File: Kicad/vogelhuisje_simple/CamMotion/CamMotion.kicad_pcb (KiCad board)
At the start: 2 copper layers, 91.4 x 137.2 mm, 20 parts, among them J6 Conn_01x21_Female, P2 GenericBoostConverter, P3 TP4056breakout, P4 TP4056breakout, Q1 Q_PMOS_GSD, U3 ESP32-LilyGo-T_PCIE, U4 PMS5003, U5 SD-card-reader, U6 BME280Breakout, U7 BME280Breakout

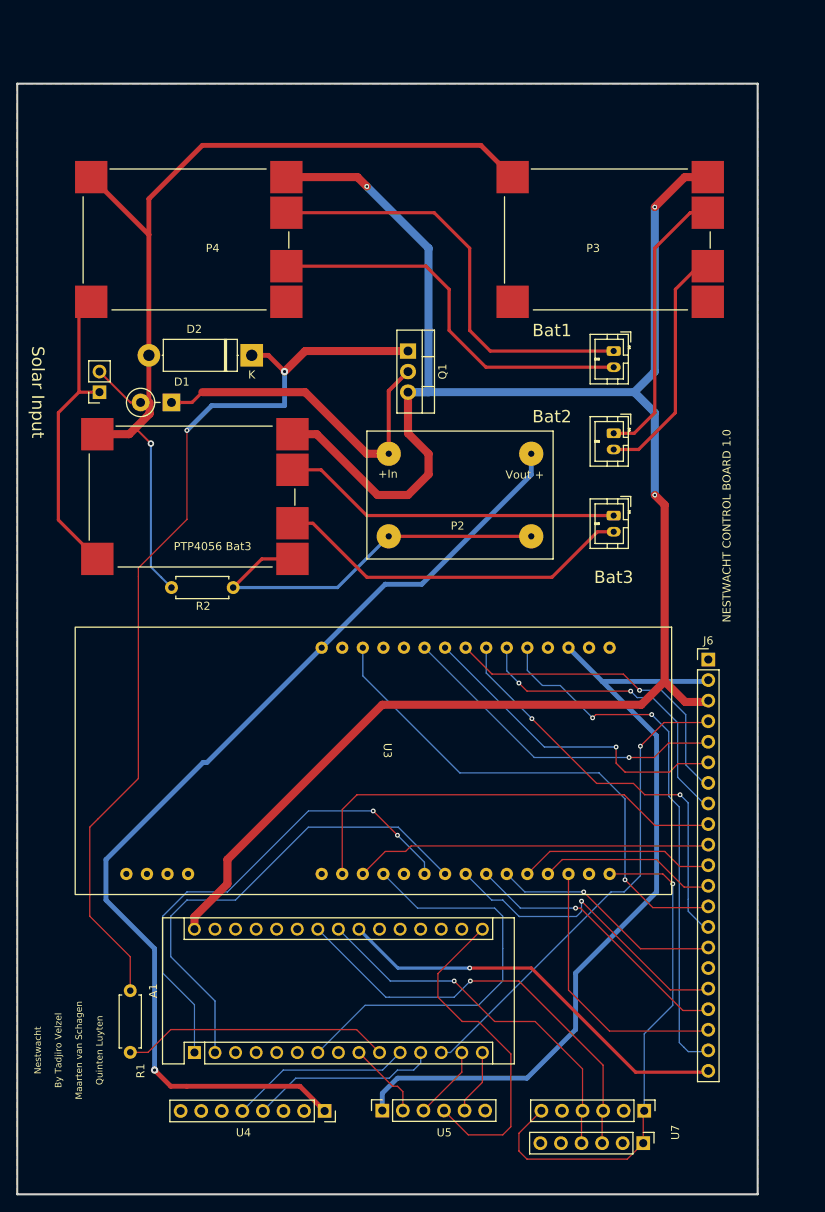
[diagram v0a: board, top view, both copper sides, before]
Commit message: Finish pcb simplified
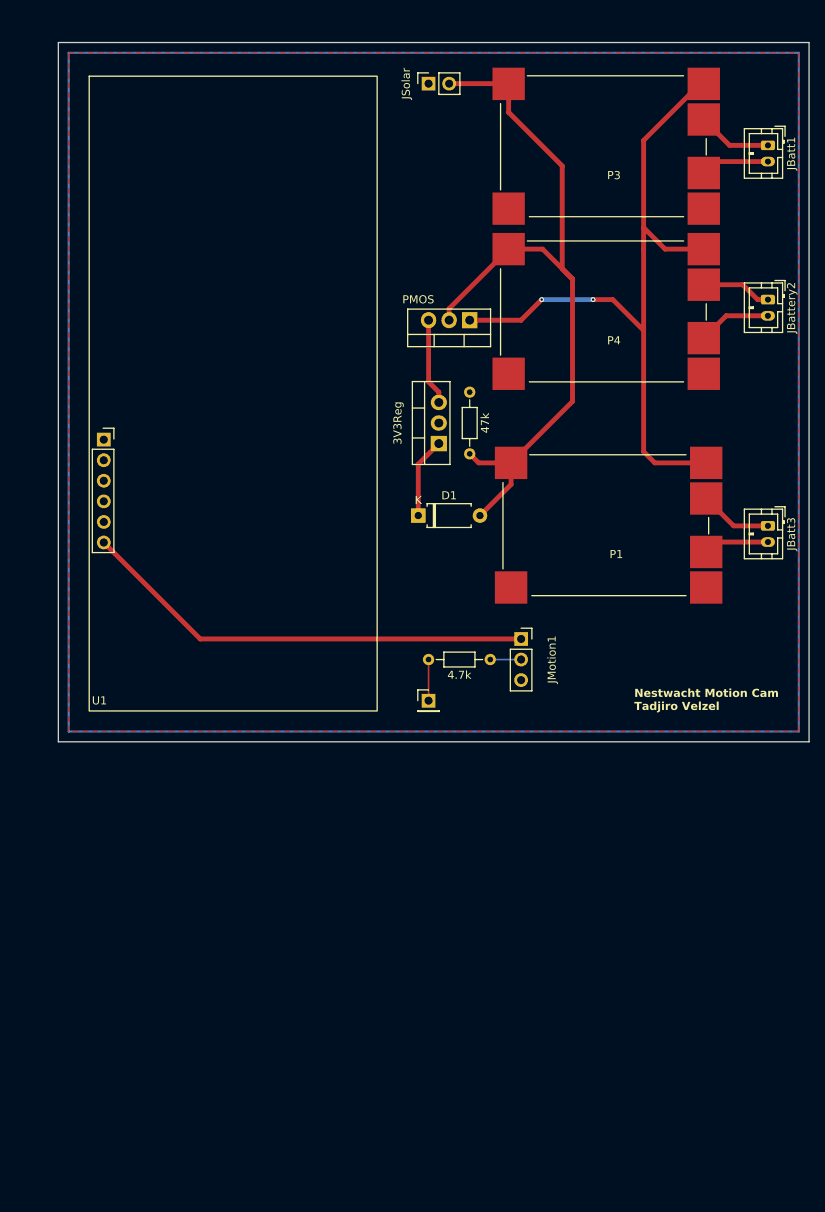
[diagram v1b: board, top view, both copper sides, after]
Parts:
- removed A1: Arduino_Nano_v3.x, Module:Arduino_Nano
- removed D2: D, Diode_THT:D_5W_P12.70mm_Horizontal
- removed J6: Conn_01x21_Female, Connector_PinHeader_2.54mm:PinHeader_1x21_P2.54mm_Vertical
- removed JSolar1: Conn_01x02_Female, Connector_PinSocket_2.54mm:PinSocket_1x02_P2.54mm_Vertical
- removed P2: GenericBoostConverter, Components:GenericBoostConverter
- removed PTP4056 Bat3: TP4056breakout, components:TP4056breakout
- removed Q1: Q_PMOS_GSD, Package_TO_SOT_THT:TO-220-3_Vertical
- removed R2: 100k, Resistor_THT:R_Axial_DIN0207_L6.3mm_D2.5mm_P7.62mm_Horizontal
- removed U3: ESP32-LilyGo-T_PCIE, components:Lilygo_T_PCIE
- removed U4: PMS5003, Connector_PinSocket_2.54mm:PinSocket_1x08_P2.54mm_Vertical
- removed U5: SD-card-reader, Connector_PinSocket_2.54mm:PinSocket_1x06_P2.54mm_Vertical
- removed U6, U7: BME280Breakout, Connector_PinHeader_2.54mm:PinHeader_1x06_P2.54mm_Vertical
- added 3V3Reg: LM3940, Package_TO_SOT_THT:TO-220-3_Vertical, F.Cu at (118.1, 87.6)
- added 47k: 47k, Resistor_THT:R_Axial_DIN0204_L3.6mm_D1.6mm_P7.62mm_Horizontal, F.Cu at (121.9, 81.3)
- added J1: Conn_01x01_Pin, Connector_PinHeader_2.54mm:PinHeader_1x01_P2.54mm_Vertical, F.Cu at (116.8, 119.4)
- added JMotion1: -, Connector_PinSocket_2.54mm:PinSocket_1x03_P2.54mm_Vertical, F.Cu at (128.3, 111.8)
- added JSolar: Conn_01x02_Female, Connector_PinSocket_2.54mm:PinSocket_1x02_P2.54mm_Vertical, F.Cu at (116.8, 43.2)
- added P1: TP4056breakout, components:TP4056breakout, F.Cu at (126.0, 106.4)
- added PMOS: Q_PMOS_DGS, Package_TO_SOT_THT:TO-220-3_Vertical, F.Cu at (121.9, 72.4)
- added U1: T-simcam, LilyGo:TSimCam, F.Cu at (74.9, 120.7)
- D1: value D_Schottky -> D_Schot; footprint Diode_THT:D_DO-41_SOD81_P3.81mm_Vertical_KathodeUp -> Diode_THT:D_A-405_P7.62mm_Horizontal
- R1: value - -> 4.7k; footprint Resistor_THT:R_Axial_DIN0207_L6.3mm_D2.5mm_P7.62mm_Horizontal -> Resistor_THT:R_Axial_DIN0204_L3.6mm_D1.6mm_P7.62mm_Horizontal
- moved R1 60.9 mm to (116.8, 114.3), turned to 0 degrees
- moved P4 52.3 mm to (125.7, 80.0)
- moved JBatt1 40.3 mm to (158.8, 50.8)
- moved D1 33.5 mm to (115.6, 96.5), turned to 0 degrees
- moved JBattery2 20.1 mm to (158.8, 69.8)
- moved JBatt3 19.1 mm to (158.8, 97.8)
- moved P3 11.5 mm to (125.7, 59.6)
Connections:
- R1 pad 1: /Sensors and microcontrollers/BOOST -> /Sensors and microcontrollers/Motion_out
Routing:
- net /Power Supply/Vbat: track 250.4 -> 89.7 mm, vias 3 -> 2
- net +5V: track 126.4 -> 0.00 mm, vias 1 -> 0
- net Net-(JMotion1-Pin_2): track 114.9 -> 3.81 mm, vias 2 -> 0
- net +3V3: track 97.8 -> 0.00 mm
- net GND: track 86.2 -> 0.00 mm
- net /Sensors and microcontrollers/PCLK_CAM: track 66.3 -> 0.00 mm, vias 2 -> 0
- net Net-(U3-Pad16): track 64.5 -> 0.00 mm, vias 1 -> 0
- net /Sensors and microcontrollers/XCLK_CAM: track 63.5 -> 0.00 mm, vias 1 -> 0
- net /Sensors and microcontrollers/TX_ARD: track 60.3 -> 0.00 mm, vias 2 -> 0
- net /Sensors and microcontrollers/RX_ARD: track 59.9 -> 0.00 mm
- net /Sensors and microcontrollers/LED_EN: track 58.8 -> 0.00 mm, vias 1 -> 0
- net Vcc: track 0.00 -> 56.5 mm
- net /Sensors and microcontrollers/Y6_CAM: track 55.1 -> 0.00 mm
- net /Sensors and microcontrollers/SCL: track 53.5 -> 0.00 mm, vias 1 -> 0
- net /Sensors and microcontrollers/INT_OUT_ARD: track 51.4 -> 0.00 mm
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- removed copper zone on B.Cu, net GND
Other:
- board size 91.4 x 137.2 mm -> 92.7 x 86.4 mm
- board text added: "Nestwacht Motion Cam Tadjiro Velzel"
- board text removed: "Bat1"
- board text removed: "Bat2"
- board text removed: "Bat3"
- board text removed: "By Tadjiro Velzel"
- board text removed: "Maarten van Schagen"
- board text removed: "NESTWACHT CONTROL BOARD 1.0"
- board text removed: "Nestwacht"
- board text removed: "Quinten Luyten"
- board text removed: "Solar Input"

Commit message: Finished PCB
Now more properly routed
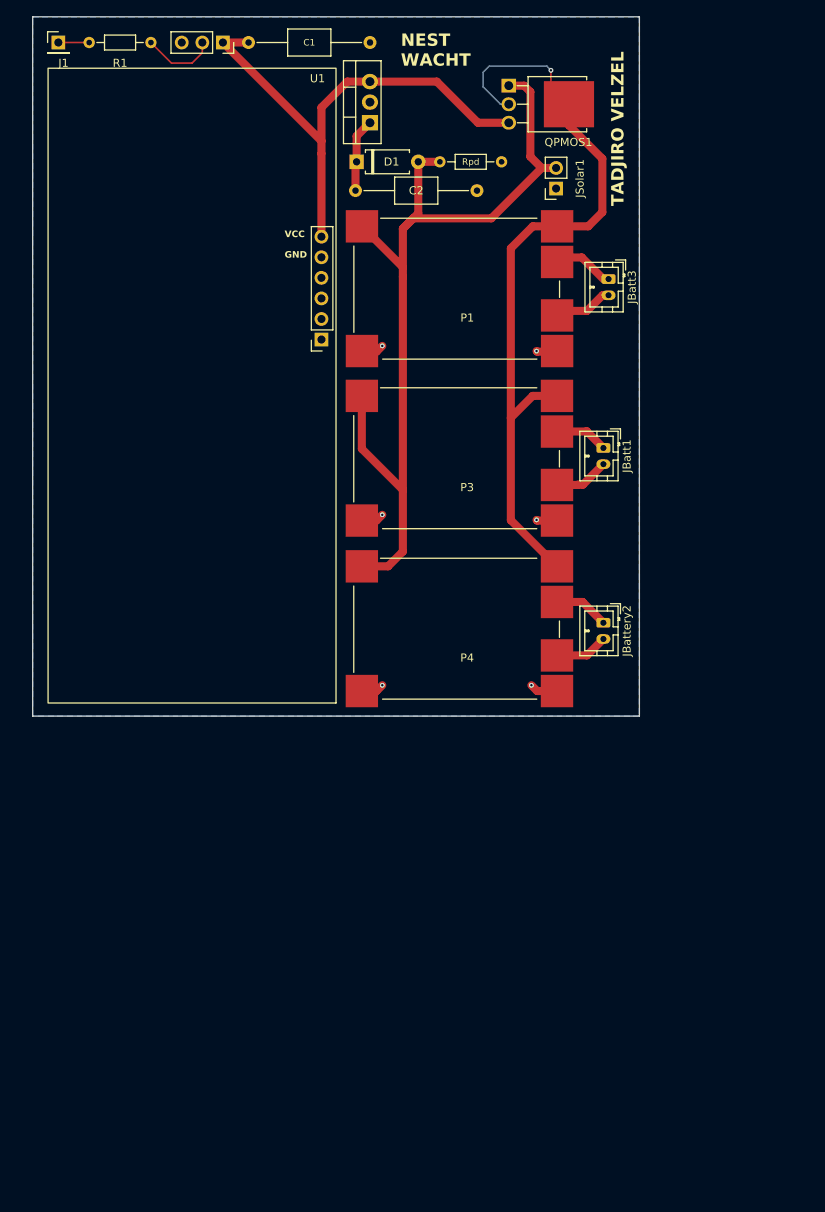
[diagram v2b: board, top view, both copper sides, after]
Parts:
- removed 3V3Reg: LM3940, Package_TO_SOT_THT:TO-220-3_Vertical
- removed 47k: 47k, Resistor_THT:R_Axial_DIN0204_L3.6mm_D1.6mm_P7.62mm_Horizontal
- removed JSolar: Conn_01x02_Female, Connector_PinSocket_2.54mm:PinSocket_1x02_P2.54mm_Vertical
- removed PMOS: Q_PMOS_DGS, Package_TO_SOT_THT:TO-220-3_Vertical
- added C1: 100u, Capacitor_THT:C_Axial_L5.1mm_D3.1mm_P15.00mm_Horizontal, F.Cu at (94.6, 38.1)
- added C2: 10u, Capacitor_THT:C_Axial_L5.1mm_D3.1mm_P15.00mm_Horizontal, F.Cu at (107.8, 56.4)
- added JSolar1: Conn_01x02_Female, Connector_PinSocket_2.54mm:PinSocket_1x02_P2.54mm_Vertical, F.Cu at (132.6, 56.1)
- added QPMOS1: TSM680P06CH, Transistors:TSM680P06CH, F.Cu at (126.7, 43.4)
- added Rpd: 47k, Resistor_THT:R_Axial_DIN0204_L3.6mm_D1.6mm_P7.62mm_Horizontal, F.Cu at (125.9, 52.8)
- added UReg1: LD1117, Package_TO_SOT_THT:TO-220-3_Vertical, F.Cu at (109.6, 48.0)
- moved J1 93.3 mm to (71.1, 38.1)
- moved R1 87.0 mm to (74.9, 38.1)
- moved U1 85.0 mm to (105.4, 41.3), turned to 180 degrees
- moved JMotion1 82.4 mm to (91.4, 38.1), turned to -90 degrees
- moved JBattery2 44.8 mm to (138.4, 109.8)
- moved D1 44.3 mm to (108.0, 52.8)
- moved P4 43.2 mm to (107.6, 119.2)
- moved P3 42.6 mm to (107.6, 98.1)
- moved JBatt1 42.5 mm to (138.4, 88.2)
- moved JBatt3 36.3 mm to (139.1, 67.3)
- moved P1 34.5 mm to (107.6, 77.2)
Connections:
- net Net-(D1-A) renamed /Power Supply/VSolar
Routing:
- net /Power Supply/VSolar: track 95.5 -> 113.3 mm
- net GND: track 0.00 -> 17.0 mm, vias 0 -> 6
- net /Power Supply/Vcc: track 10.7 -> 0.00 mm
- net /Power Supply/Vbat: track 89.7 -> 96.5 mm, vias 2 -> 1
- net Vcc: track 56.5 -> 62.9 mm
- net Net-(JMotion1-Pin_2): track 3.81 -> 9.20 mm
- net Net-(JBatt1-Pin_1): track 9.24 -> 6.60 mm
- net Net-(JBattery2-Pin_2): track 9.06 -> 6.57 mm
- net Net-(JBatt3-Pin_1): track 9.02 -> 6.83 mm
- net Net-(JBattery2-Pin_1): track 8.68 -> 6.79 mm
- net Net-(JBatt1-Pin_2): track 8.50 -> 6.79 mm
- net Net-(JBatt3-Pin_2): track 8.13 -> 6.53 mm
- net /Sensors and microcontrollers/Motion_out: track 5.08 -> 3.81 mm
- net Net-(D1-K): track 9.94 -> 9.12 mm
- added copper zone on B.Cu, net GND
- removed copper zone on F.Cu, net GND
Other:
- board size 92.7 x 86.4 mm -> 74.9 x 86.4 mm
- board text added: "GND"
- board text added: "NEST WACHT"
- board text added: "TADJIRO VELZEL"
- board text added: "VCC"
- board text removed: "Nestwacht Motion Cam Tadjiro Velzel"
